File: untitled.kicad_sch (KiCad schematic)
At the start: 4 parts, among them J1 Conn_01x04_Male, J2 Conn_01x09_Male, J3 Conn_01x04_Male, J4 Conn_02x03_Odd_Even

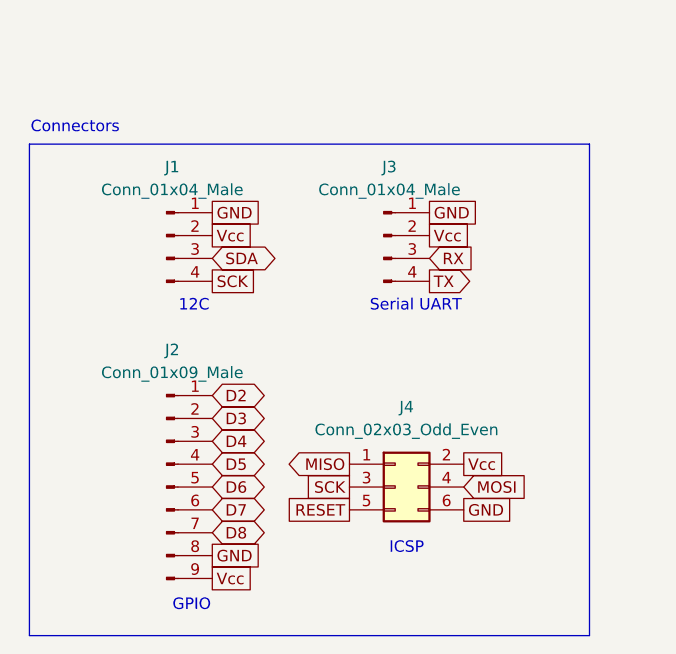
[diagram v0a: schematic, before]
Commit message: Initial commit - The MCU datalogger
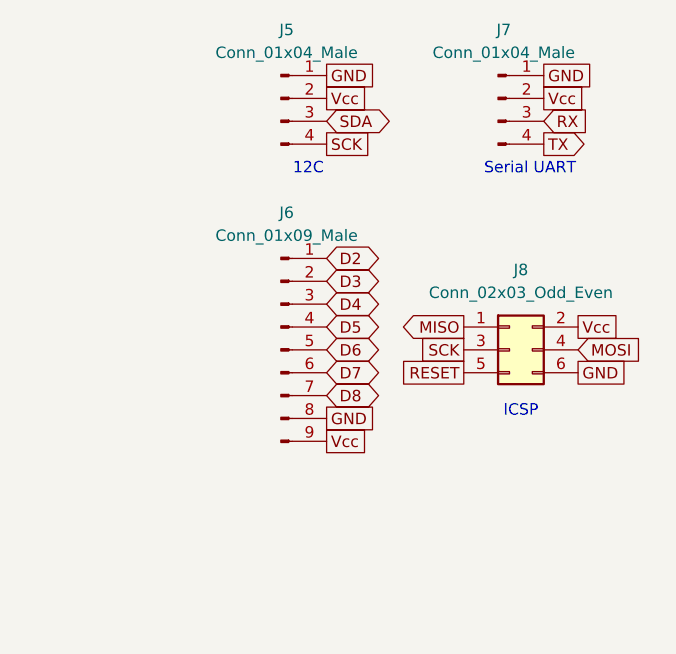
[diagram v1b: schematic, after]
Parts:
- removed J1, J3: Conn_01x04_Male, Connector_PinHeader_2.54mm:PinHeader_1x04_P2.54mm_Vertical, symbol Connector:Conn_01x04_Pin
- removed J2: Conn_01x09_Male, Connector_PinHeader_2.54mm:PinHeader_1x09_P2.54mm_Vertical, symbol Connector:Conn_01x09_Pin
- removed J4: Conn_02x03_Odd_Even, Connector_PinHeader_2.54mm:PinHeader_2x03_P2.54mm_Vertical, symbol Connector_Generic:Conn_02x03_Odd_Even
- added J5, J7: Conn_01x04_Male, Connector_PinHeader_2.54mm:PinHeader_1x04_P2.54mm_Vertical, symbol Connector:Conn_01x04_Pin
- added J6: Conn_01x09_Male, Connector_PinHeader_2.54mm:PinHeader_1x09_P2.54mm_Vertical, symbol Connector:Conn_01x09_Pin
- added J8: Conn_02x03_Odd_Even, Connector_PinHeader_2.54mm:PinHeader_2x03_P2.54mm_Vertical, symbol Connector_Generic:Conn_02x03_Odd_Even
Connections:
- net D2: now also J6.1 (Pin_1)
- net D3: now also J6.2 (Pin_2)
- net D4: now also J6.3 (Pin_3)
- net D5: now also J6.4 (Pin_4)
- net D6: now also J6.5 (Pin_5)
- net D7: now also J6.6 (Pin_6)
- net D8: now also J6.7 (Pin_7)
- net GND: now also J5.1 (Pin_1), J6.8 (Pin_8), J7.1 (Pin_1), J8.6 (Pin_6)
- net MISO: now also J8.1 (Pin_1)
- net MOSI: now also J8.4 (Pin_4)
- net RESET: now also J8.5 (Pin_5)
- net RX: now also J7.3 (Pin_3)
- net SCK: now also J5.4 (Pin_4), J8.3 (Pin_3)
- net SDA: now also J5.3 (Pin_3)
- net TX: now also J7.4 (Pin_4)
- net Vcc: now also J5.2 (Pin_2), J6.9 (Pin_9), J7.2 (Pin_2), J8.2 (Pin_2)
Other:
- note removed: "Connectors"
- note removed: "GPIO"
